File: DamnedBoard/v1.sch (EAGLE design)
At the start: 17 parts, among them U1 EFM32ZG108, U2 MAX44009EDT+T21-0490D-M

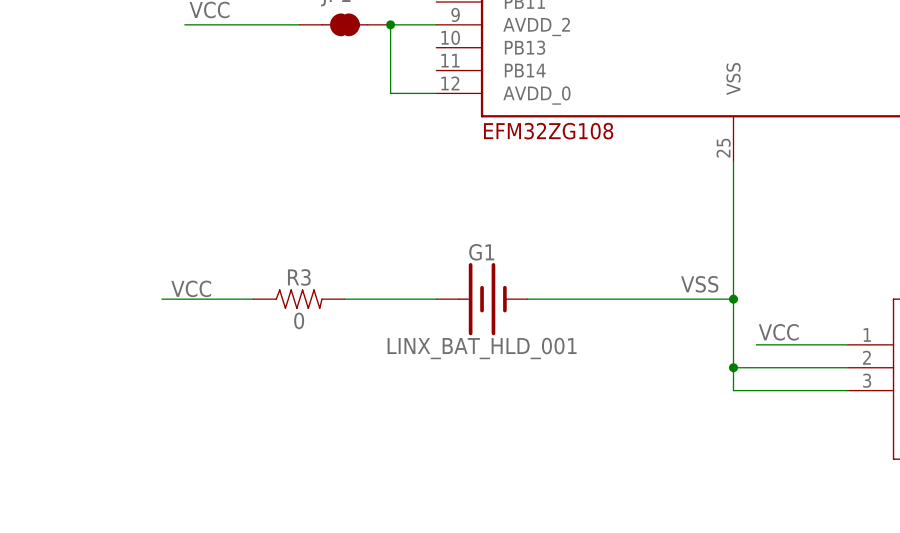
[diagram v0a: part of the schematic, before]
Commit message: OSH Parkifying layout.
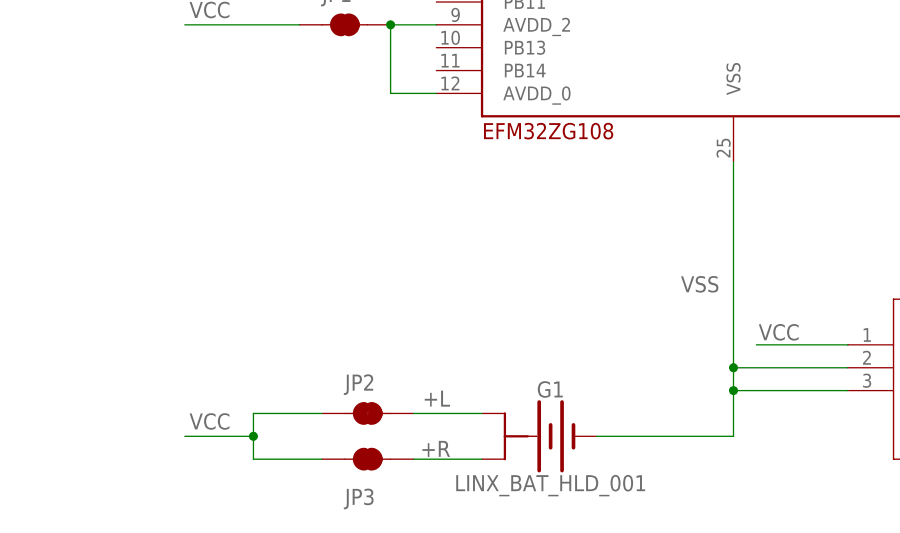
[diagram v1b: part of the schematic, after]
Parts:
- removed R3: 0, SparkFun-Resistors:0OHM-0603-1/10W-5%
- added JP2, JP3: JUMPER-SMT_2_NC_TRACE_NO-SILK, SparkFun-Jumpers:JUMPER-SMT_2_NC_TRACE_NO-SILK
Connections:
- removed net N$1: G1.+, R3.2
- new net +L: G1.+$1, JP2.2
- new net +R: G1.+$2, JP3.2
- net VCC: now also JP2.1, JP3.1; no longer R3.1
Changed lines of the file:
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@@
 <parts>
 <part name="TC1" library="TagConnect" deviceset="TC2050-IDC" device=""/>
-<part name="G1" library="boneyard" deviceset="LINX_BAT_HLD_001" device="" package3d_urn="urn:adsk.eagle:package:291704/2"/>
 <part name="U2" library="boneyard" deviceset="MAX44009EDT+T" device="21-0490D-M" package3d_urn="urn:adsk.eagle:package:291621/2"/>
 <part name="U1" library="boneyard" deviceset="EFM32ZG108" device=""/>
@@
 <part name="R2" library="SparkFun-Resistors" library_urn="urn:adsk.eagle:library:532" deviceset="68OHM" device="-0603-1/10W-1%" package3d_urn="urn:adsk.eagle:package:39650/1"/>
 <part name="U$1" library="boneyard" deviceset="DAMNED" device=""/>
-<part name="R3" library="SparkFun-Resistors" library_urn="urn:adsk.eagle:library:532" deviceset="0OHM" device="-0603-1/10W-5%" package3d_urn="urn:adsk.eagle:package:39650/1" value="0"/>
 <part name="C1" library="SparkFun-Capacitors" library_urn="urn:adsk.eagle:library:510" deviceset="1.0UF" device="-0603-16V-10%" package3d_urn="urn:adsk.eagle:package:37414/1" value="1.0uF"/>
 <part name="JP1" library="SparkFun-Jumpers" library_urn="urn:adsk.eagle:library:528" deviceset="JUMPER-SMT_2_NC_TRACE" device="_NO-SILK" package3d_urn="urn:adsk.eagle:package:39286/1"/>
@@
 <part name="C5" library="SparkFun-Capacitors" library_urn="urn:adsk.eagle:library:510" deviceset="0.1UF" device="-0402-16V-10%" package3d_urn="urn:adsk.eagle:package:37413/1" value="0.1uF"/>
 <part name="C6" library="SparkFun-Capacitors" library_urn="urn:adsk.eagle:library:510" deviceset="10UF" device="-0603-6.3V-20%" package3d_urn="urn:adsk.eagle:package:37414/1" value="10uF"/>
+<part name="G1" library="boneyard" deviceset="LINX_BAT_HLD_001" device="" package3d_urn="urn:adsk.eagle:package:291704/2"/>
+<part name="JP2" library="SparkFun-Jumpers" library_urn="urn:adsk.eagle:library:528" deviceset="JUMPER-SMT_2_NC_TRACE" device="_NO-SILK" package3d_urn="urn:adsk.eagle:package:39286/1"/>
+<part name="JP3" library="SparkFun-Jumpers" library_urn="urn:adsk.eagle:library:528" deviceset="JUMPER-SMT_2_NC_TRACE" device="_NO-SILK" package3d_urn="urn:adsk.eagle:package:39286/1"/>
 </parts>
 <sheets>
@@
 <instances>
 <instance part="TC1" gate="A" x="-27.94" y="50.8" rot="R180"/>
-<instance part="G1" gate="G$1" x="43.18" y="27.94"/>
 <instance part="U2" gate="A" x="86.36" y="22.86"/>
 <instance part="U1" gate="G$1" x="55.88" y="55.88"/>
@@
 </instance>
 <instance part="U$1" gate="G$1" x="48.26" y="104.14"/>
-<instance part="R3" gate="G$1" x="27.94" y="27.94"/>
 <instance part="C1" gate="G$1" x="142.24" y="63.5"/>
 <instance part="JP1" gate="G$1" x="33.02" y="58.42" smashed="yes">
@@
 <instance part="C5" gate="G$1" x="17.78" y="71.12"/>
 <instance part="C6" gate="G$1" x="5.08" y="71.12"/>
+<instance part="G1" gate="G$1" x="50.8" y="12.7"/>
+<instance part="JP2" gate="G$1" x="35.56" y="15.24" smashed="yes">
+<attribute name="NAME" x="33.02" y="17.78" size="1.778" layer="95" font="vector"/>
+</instance>
+<instance part="JP3" gate="G$1" x="35.56" y="10.16" smashed="yes">
+<attribute name="NAME" x="33.02" y="5.08" size="1.778" layer="95" font="vector"/>
+</instance>
 </instances>
 <busses>
@@
 <net name="VSS" class="0">
 <segment>
-<pinref part="G1" gate="G$1" pin="-"/>
 <pinref part="U1" gate="G$1" pin="VSS"/>
-<wire x1="53.34" y1="27.94" x2="76.2" y2="27.94" width="0.1524" layer="91"/>
-<wire x1="76.2" y1="27.94" x2="76.2" y2="43.18" width="0.1524" layer="91"/>
+<wire x1="76.2" y1="20.32" x2="76.2" y2="43.18" width="0.1524" layer="91"/>
 <pinref part="U2" gate="A" pin="GND"/>
 <wire x1="88.9" y1="20.32" x2="76.2" y2="20.32" width="0.1524" layer="91"/>
-<wire x1="76.2" y1="20.32" x2="76.2" y2="27.94" width="0.1524" layer="91"/>
-<junction x="76.2" y="27.94"/>
 <pinref part="U2" gate="A" pin="A0"/>
 <wire x1="88.9" y1="17.78" x2="76.2" y2="17.78" width="0.1524" layer="91"/>
@@
 <junction x="76.2" y="20.32"/>
 <label x="70.358" y="28.702" size="1.778" layer="95"/>
+<pinref part="G1" gate="G$1" pin="-"/>
+<wire x1="60.96" y1="12.7" x2="76.2" y2="12.7" width="0.1524" layer="91"/>
+<wire x1="76.2" y1="12.7" x2="76.2" y2="17.78" width="0.1524" layer="91"/>
+<junction x="76.2" y="17.78"/>
 </segment>
 <segment>
@@
 </segment>
 <segment>
-<pinref part="R3" gate="G$1" pin="1"/>
-<wire x1="22.86" y1="27.94" x2="12.7" y2="27.94" width="0.1524" layer="91"/>
-<label x="13.716" y="28.194" size="1.778" layer="95"/>
-</segment>
-<segment>
 <pinref part="TC1" gate="A" pin="1"/>
 <wire x1="-35.56" y1="55.88" x2="-43.18" y2="55.88" width="0.1524" layer="91"/>
@@
 <pinref part="C3" gate="G$1" pin="2"/>
 </segment>
+<segment>
+<pinref part="JP2" gate="G$1" pin="1"/>
+<wire x1="30.48" y1="15.24" x2="22.86" y2="15.24" width="0.1524" layer="91"/>
+<wire x1="22.86" y1="15.24" x2="22.86" y2="12.7" width="0.1524" layer="91"/>
+<wire x1="22.86" y1="12.7" x2="15.24" y2="12.7" width="0.1524" layer="91"/>
+<pinref part="JP3" gate="G$1" pin="1"/>
+<wire x1="30.48" y1="10.16" x2="22.86" y2="10.16" width="0.1524" layer="91"/>
+<wire x1="22.86" y1="10.16" x2="22.86" y2="12.7" width="0.1524" layer="91"/>
+<junction x="22.86" y="12.7"/>
+<label x="15.748" y="13.462" size="1.778" layer="95"/>
+</segment>
 </net>
 <net name="PA0" class="0">
@@
 <pinref part="D2" gate="G$1" pin="C"/>
 <wire x1="-17.78" y1="99.06" x2="-17.78" y2="86.36" width="0.1524" layer="91"/>
-</segment>
-</net>
-<net name="N$1" class="0">
-<segment>
-<pinref part="G1" gate="G$1" pin="+"/>
-<pinref part="R3" gate="G$1" pin="2"/>
-<wire x1="43.18" y1="27.94" x2="33.02" y2="27.94" width="0.1524" layer="91"/>
 </segment>
 </net>
@@
 </segment>
 </net>
+<net name="+R" class="0">
+<segment>
+<pinref part="G1" gate="G$1" pin="+$2"/>
+<pinref part="JP3" gate="G$1" pin="2"/>
+<wire x1="48.26" y1="10.16" x2="40.64" y2="10.16" width="0.1524" layer="91"/>
+<label x="41.402" y="10.414" size="1.778" layer="95"/>
+</segment>
+</net>
+<net name="+L" class="0">
+<segment>
+<pinref part="G1" gate="G$1" pin="+$1"/>
+<pinref part="JP2" gate="G$1" pin="2"/>
+<wire x1="48.26" y1="15.24" x2="40.64" y2="15.24" width="0.1524" layer="91"/>
+<label x="41.656" y="16.002" size="1.778" layer="95"/>
+</segment>
+</net>
